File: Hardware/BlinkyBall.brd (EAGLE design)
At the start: 3 parts, among them IC3 TINY13-20SSU

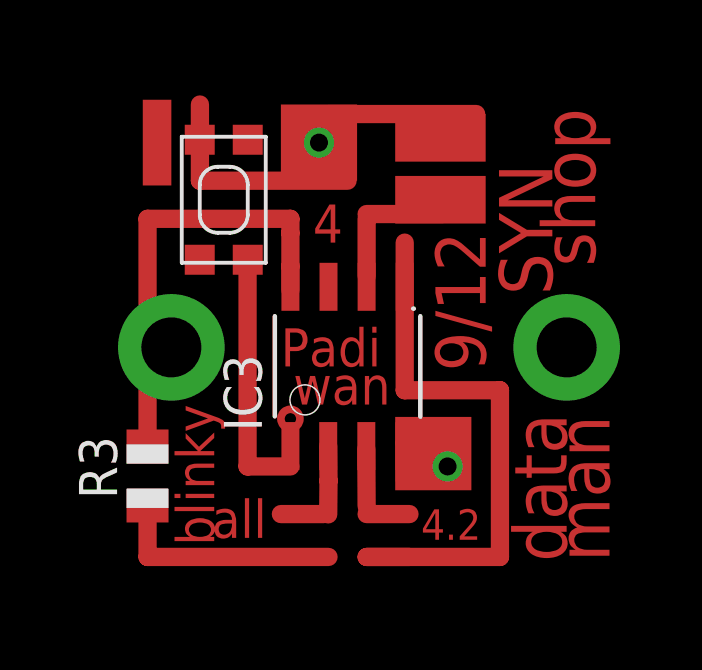
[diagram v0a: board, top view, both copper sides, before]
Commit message: Final Board Adjustments?
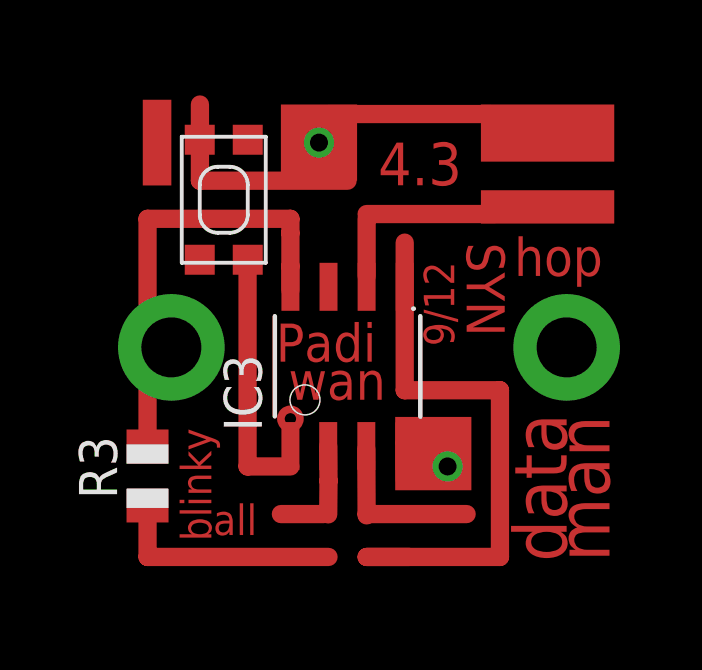
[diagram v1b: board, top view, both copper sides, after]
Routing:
- net S$2: track 6.35 -> 8.73 mm
- net S$5: track 2.54 -> 4.29 mm
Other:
- board text added: "4.3"
- board text added: "hop"
- board text removed: "4"
- board text removed: "4.2"
- board text removed: "shop"
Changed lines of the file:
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@@
 <plain>
 <circle x="8.09625" y="7.62" radius="0.3175" width="0.254" layer="1"/>
-<text x="14.605" y="9.2075" size="1.6764" layer="1" rot="R90">9/12</text>
 <rectangle x1="7.77875" y1="15.5575" x2="10.31875" y2="18.0975" layer="1"/>
 <rectangle x1="11.58875" y1="5.23875" x2="14.12875" y2="7.6835" layer="1"/>
-<rectangle x1="11.58875" y1="16.1925" x2="14.605" y2="17.78" layer="1"/>
-<rectangle x1="11.58875" y1="14.12875" x2="14.605" y2="15.71625" layer="1"/>
-<text x="16.8275" y="11.7475" size="1.778" layer="1" rot="R90">SYN</text>
 <text x="18.7325" y="2.8575" size="1.778" layer="1" rot="R90">man</text>
-<text x="4.28625" y="8.09625" size="1.27" layer="1" rot="R270">blinky</text>
-<text x="7.3025" y="4.92125" size="1.27" layer="1" rot="R180">all</text>
-<text x="14.44625" y="4.60375" size="1.016" layer="1" rot="R180">4.2</text>
-<text x="18.25625" y="12.7" size="1.778" layer="1" rot="R90">shop</text>
+<text x="4.445" y="7.3025" size="1.016" layer="1" rot="R270">blinky</text>
+<text x="6.985" y="4.7625" size="1.016" layer="1" rot="R180">all</text>
+<text x="13.81125" y="16.8275" size="1.4224" layer="1" rot="R180">4.3</text>
 <text x="17.30375" y="2.8575" size="1.778" layer="1" rot="R90">data</text>
-<text x="11.1125" y="10.63625" size="1.27" layer="1" rot="R180">Padi</text>
-<text x="11.43" y="9.36625" size="1.27" layer="1" rot="R180">wan</text>
-<text x="9.8425" y="14.76375" size="1.27" layer="1" rot="R180">4</text>
+<text x="10.95375" y="10.795" size="1.27" layer="1" rot="R180">Padi</text>
+<text x="11.27125" y="9.525" size="1.27" layer="1" rot="R180">wan</text>
 <rectangle x1="3.175" y1="15.39875" x2="4.1275" y2="18.25625" layer="1"/>
+<rectangle x1="14.44625" y1="16.1925" x2="18.89125" y2="18.0975" layer="1"/>
+<text x="13.97" y="13.49375" size="1.27" layer="1" rot="SR270">SYN</text>
+<text x="15.5575" y="12.3825" size="1.27" layer="1">hop</text>
+<text x="12.54125" y="12.85875" size="1.016" layer="1" rot="R270">9/12</text>
+<rectangle x1="14.44625" y1="14.12875" x2="18.89125" y2="15.24" layer="1"/>
 </plain>
 <attributes>
@@
 <contactref element="IC3" pad="3"/>
 <wire x1="10.62625" y1="6.71225" x2="10.62625" y2="6.61375" width="0.4064" layer="1"/>
-<wire x1="10.62625" y1="6.61375" x2="10.63625" y2="4.71875" width="0.6096" layer="1"/>
+<wire x1="10.62625" y1="6.61375" x2="10.63625" y2="4.40125" width="0.6096" layer="1"/>
 </signal>
 <signal name="N$28">
@@
 </signal>
 <signal name="S$2">
-<wire x1="10.63625" y1="4.445" x2="12.065" y2="4.445" width="0.6096" layer="1"/>
-<wire x1="9.36625" y1="17.78" x2="14.2875" y2="17.78" width="0.6096" layer="1"/>
+<wire x1="10.63625" y1="4.445" x2="13.97" y2="4.445" width="0.6096" layer="1"/>
+<wire x1="9.36625" y1="17.78" x2="14.76375" y2="17.78" width="0.6096" layer="1"/>
 </signal>
 <signal name="S$3">
@@
 </signal>
 <signal name="S$5">
-<wire x1="10.63625" y1="14.44625" x2="13.17625" y2="14.44625" width="0.6096" layer="1"/>
+<wire x1="10.63625" y1="14.44625" x2="14.9225" y2="14.44625" width="0.6096" layer="1"/>
 </signal>
 <signal name="S$6">
